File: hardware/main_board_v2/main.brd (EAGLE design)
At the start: 86.4 x 67.5 mm, 59 parts, among them IC2 LM2937, Q1 8MHz, U2 STM32F103C6T6A, U3 LSM9DS0, X1 MINI-USB-32005-201

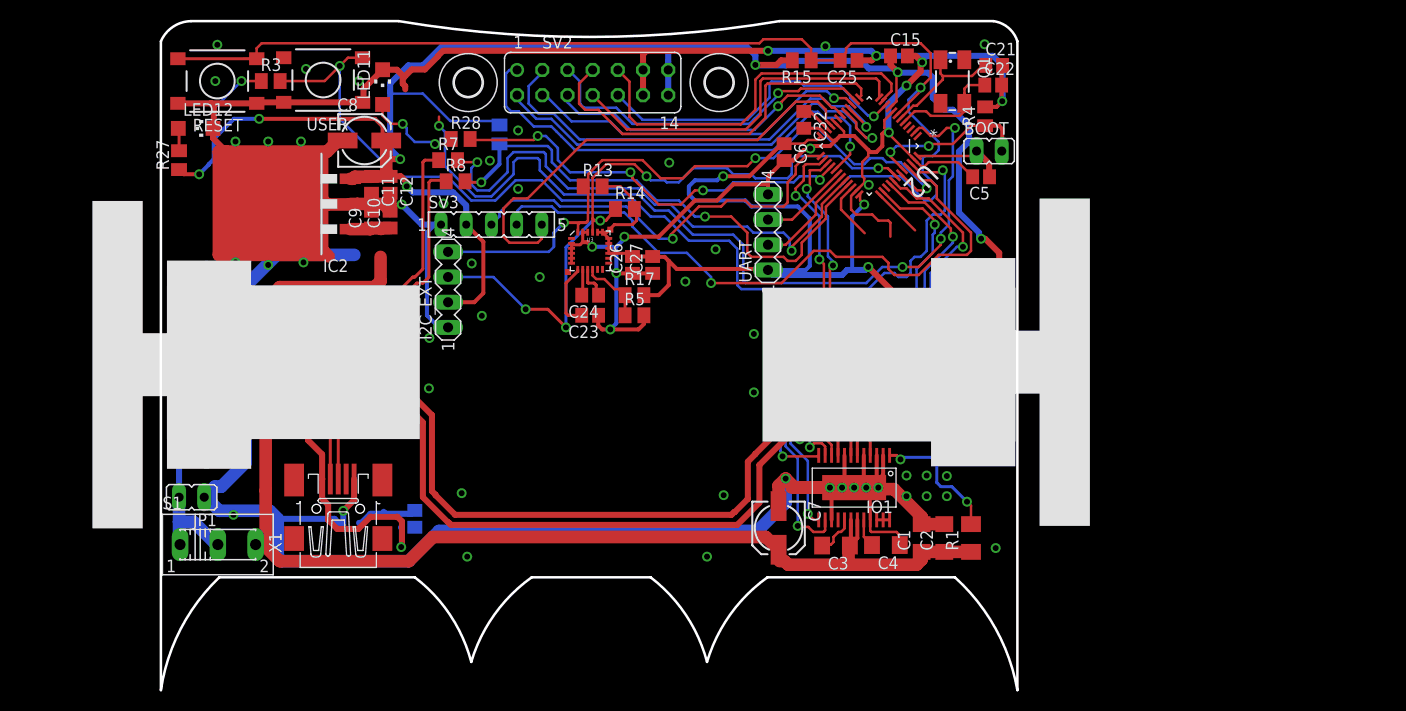
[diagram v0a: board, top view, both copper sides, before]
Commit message: common
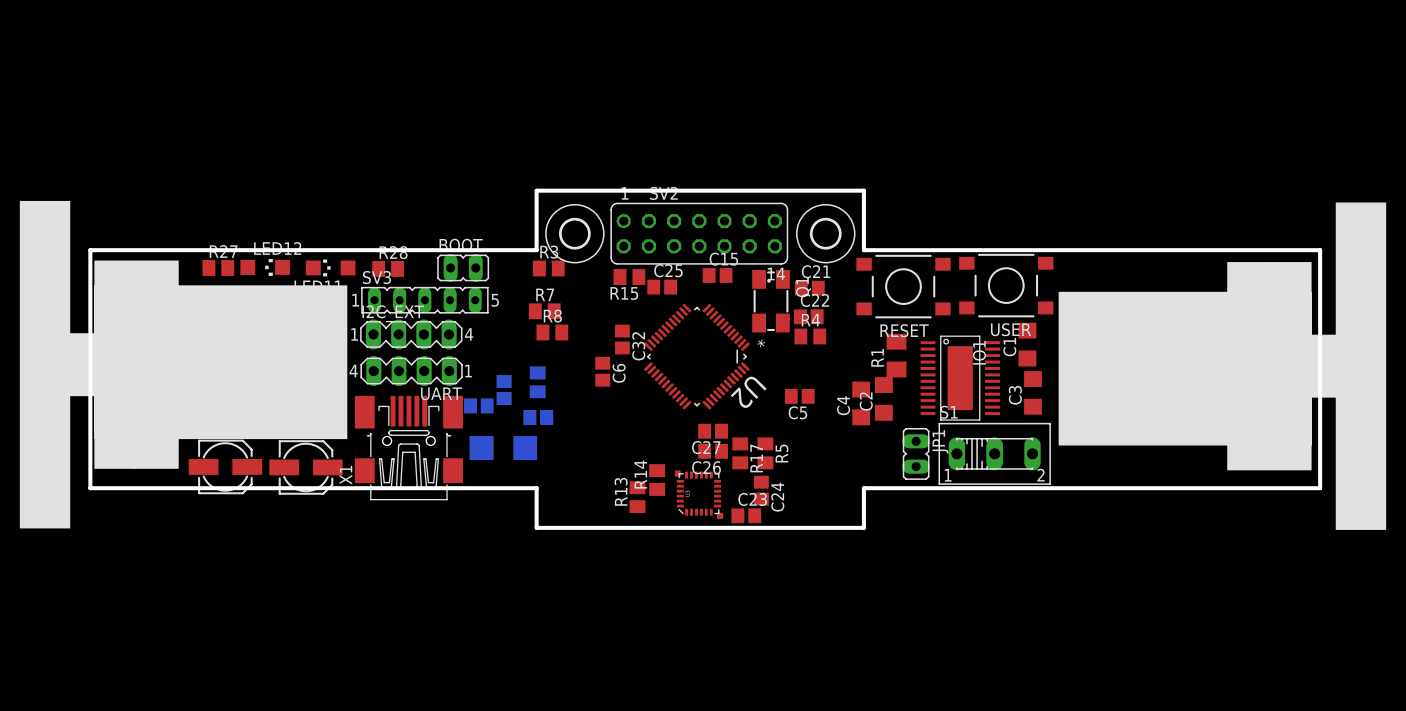
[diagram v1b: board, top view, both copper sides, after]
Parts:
- moved S1 78.9 mm to (91.2, 13.5)
- moved JP1 73.2 mm to (83.3, 13.5), turned to 180 degrees
- moved RESET 72.2 mm to (82.0, 30.3)
- moved USER 71.9 mm to (92.4, 30.4)
- moved BOOT 54.3 mm to (37.6, 32.2)
- moved C7 48.0 mm to (21.7, 12.1), turned to 0 degrees
- moved UART 38.6 mm to (32.4, 21.8), turned to 180 degrees
- moved C8 35.8 mm to (13.6, 12.1)
- moved R3 33.8 mm to (46.2, 32.2)
- moved R13 31.7 mm to (55.2, 9.09), turned to 90 degrees
- moved U$1 29.9 mm to (97.6, 22.3)
- moved C22 29.9 mm to (72.4, 27.3)
- moved C25 29.6 mm to (57.7, 30.3), turned to 0 degrees
- moved C21 29.2 mm to (72.5, 30.2)
- moved C5 28.7 mm to (71.5, 19.3)
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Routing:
- net GND: track 479.8 -> 0.00 mm, vias 81 -> 0
- net +3V3: track 307.5 -> 0.00 mm, vias 11 -> 0
- net VCC: track 128.8 -> 0.00 mm
- net RESET: track 116.0 -> 0.00 mm, vias 1 -> 0
- net USER_KEY_1: track 100.6 -> 0.00 mm, vias 2 -> 0
- net SERVO: track 85.7 -> 0.00 mm, vias 4 -> 0
- net SCL: track 71.7 -> 0.00 mm, vias 5 -> 0
- net N$4: track 71.1 -> 0.00 mm
- net SDA: track 67.3 -> 0.00 mm, vias 3 -> 0
- net CAM_CLK: track 66.8 -> 0.00 mm, vias 1 -> 0
- net N$3: track 61.0 -> 0.00 mm
- net USBDM: track 54.3 -> 0.00 mm, vias 2 -> 0
- net USBDP: track 53.0 -> 0.00 mm, vias 2 -> 0
- net M1: track 52.6 -> 0.00 mm, vias 2 -> 0
- net APHASE: track 50.2 -> 0.00 mm, vias 2 -> 0
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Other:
- board size 86.4 x 67.5 mm -> 124 x 34 mm

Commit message: debug app added
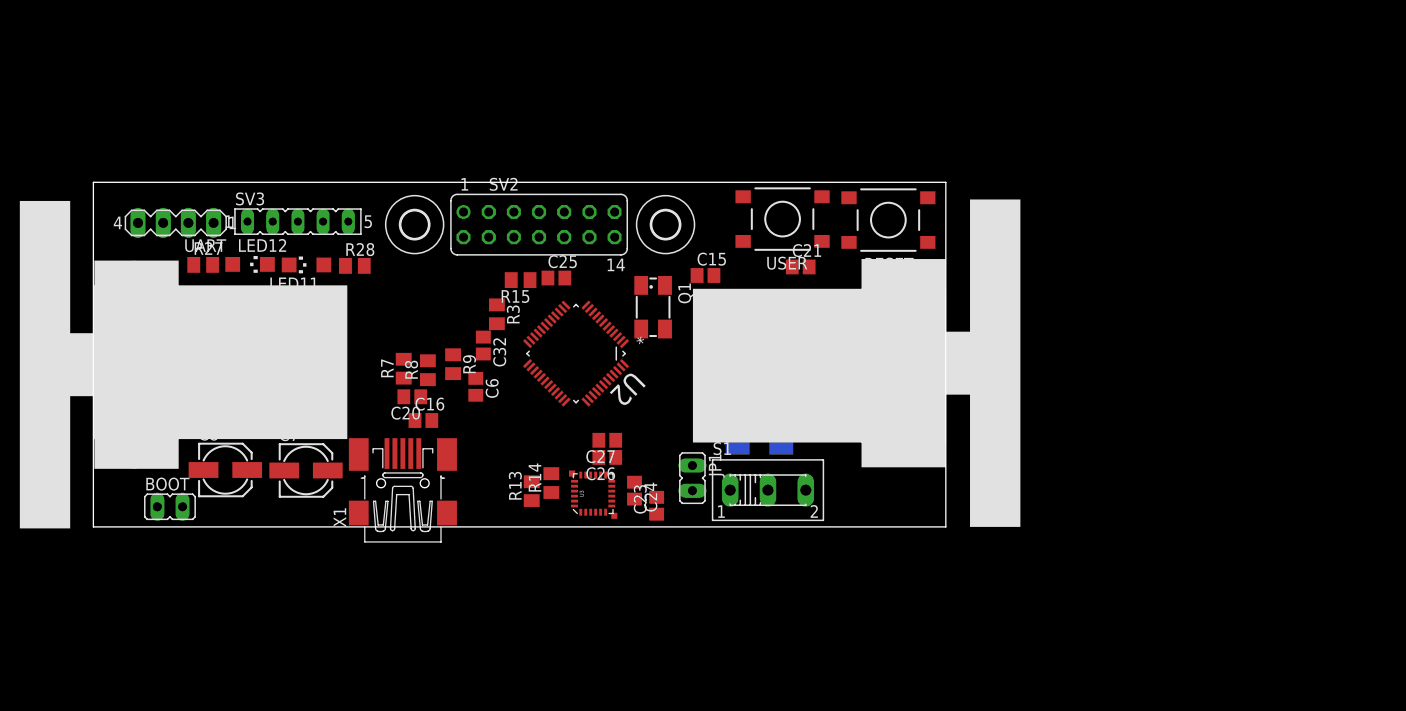
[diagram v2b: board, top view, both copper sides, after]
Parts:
- removed C13: 10uF, resistor:C0805
- removed I2C_EXT: (no value), con-lstb:MA04-1
- removed R17, R5: 47k, resistor:M0805
- moved BOOT 38.1 mm to (8.03, 8.13)
- moved U$1 36.9 mm to (60.8, 22.6)
- moved UART 28.1 mm to (8.61, 36.7)
- moved D1 25.8 mm to (67.5, 14.6), turned to 0 degrees
- moved USER 23.5 mm to (69.8, 37.1)
- moved S1 23.2 mm to (68.3, 9.80)
- moved JP1 22.7 mm to (60.7, 11.0)
- moved IO1 20.9 mm to (66.8, 22.5), flipped to the bottom, turned to 90 degrees
- moved C3 20.4 mm to (74.9, 22.8), turned to 180 degrees
- moved C1 17.5 mm to (77.1, 26.9)
- moved H1 16.2 mm to (32.7, 36.6)
- moved H2 16.2 mm to (58.0, 36.6)
- moved SV2 16.2 mm to (45.2, 36.6)
- moved R7 15.4 mm to (31.6, 22.0), turned to 90 degrees
- moved SV3 15.1 mm to (20.9, 36.9)
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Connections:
- removed net N$18: R17.1, R5.1, U3.10
- removed net SERVO: U2.2
- net +3V3: no longer I2C_EXT.2, R17.2, SV2.13
- net GND: no longer C13.2, I2C_EXT.1, R5.2, SV2.11
- net N$57: no longer C13.1
- net SCL: no longer I2C_EXT.3
- net SDA: no longer I2C_EXT.4
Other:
- board size 124 x 34 mm -> 86 x 34.7 mm
